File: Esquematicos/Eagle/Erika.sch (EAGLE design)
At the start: 12 parts

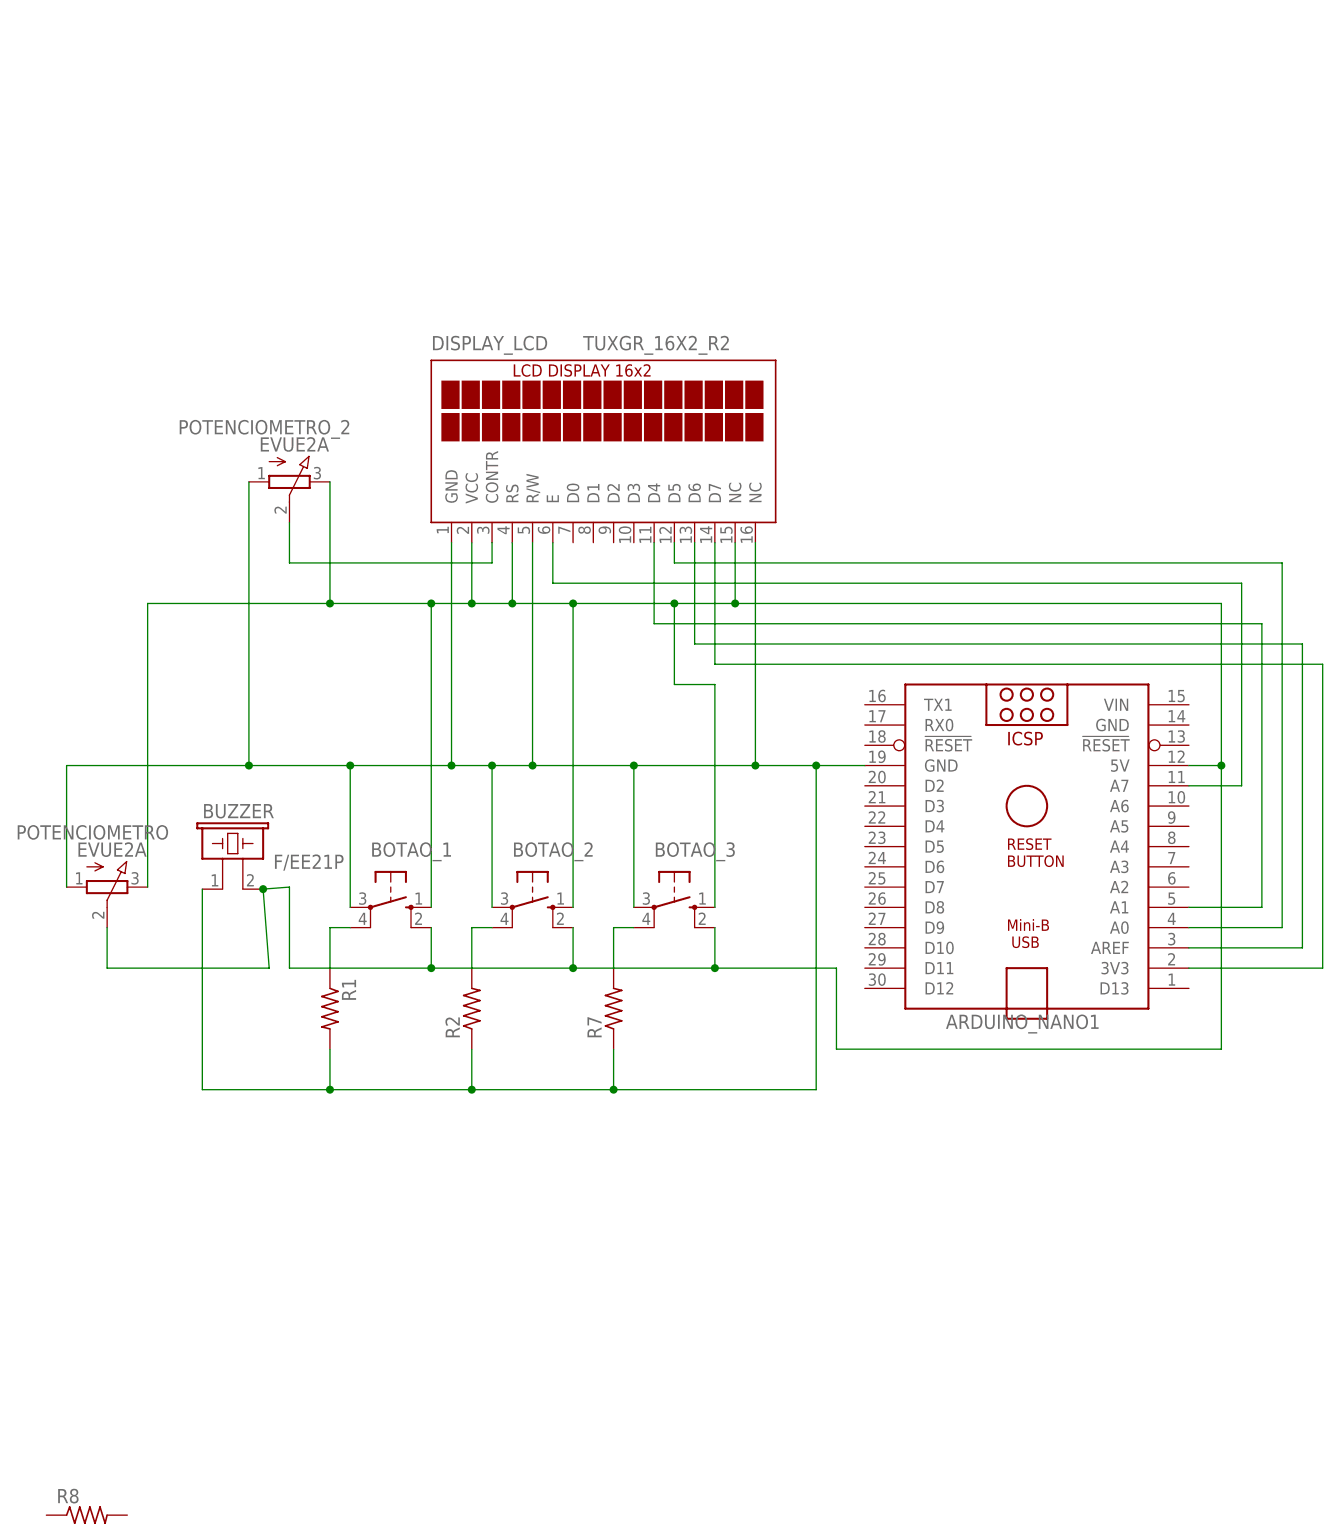
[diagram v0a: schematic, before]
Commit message: Correção do esquemático
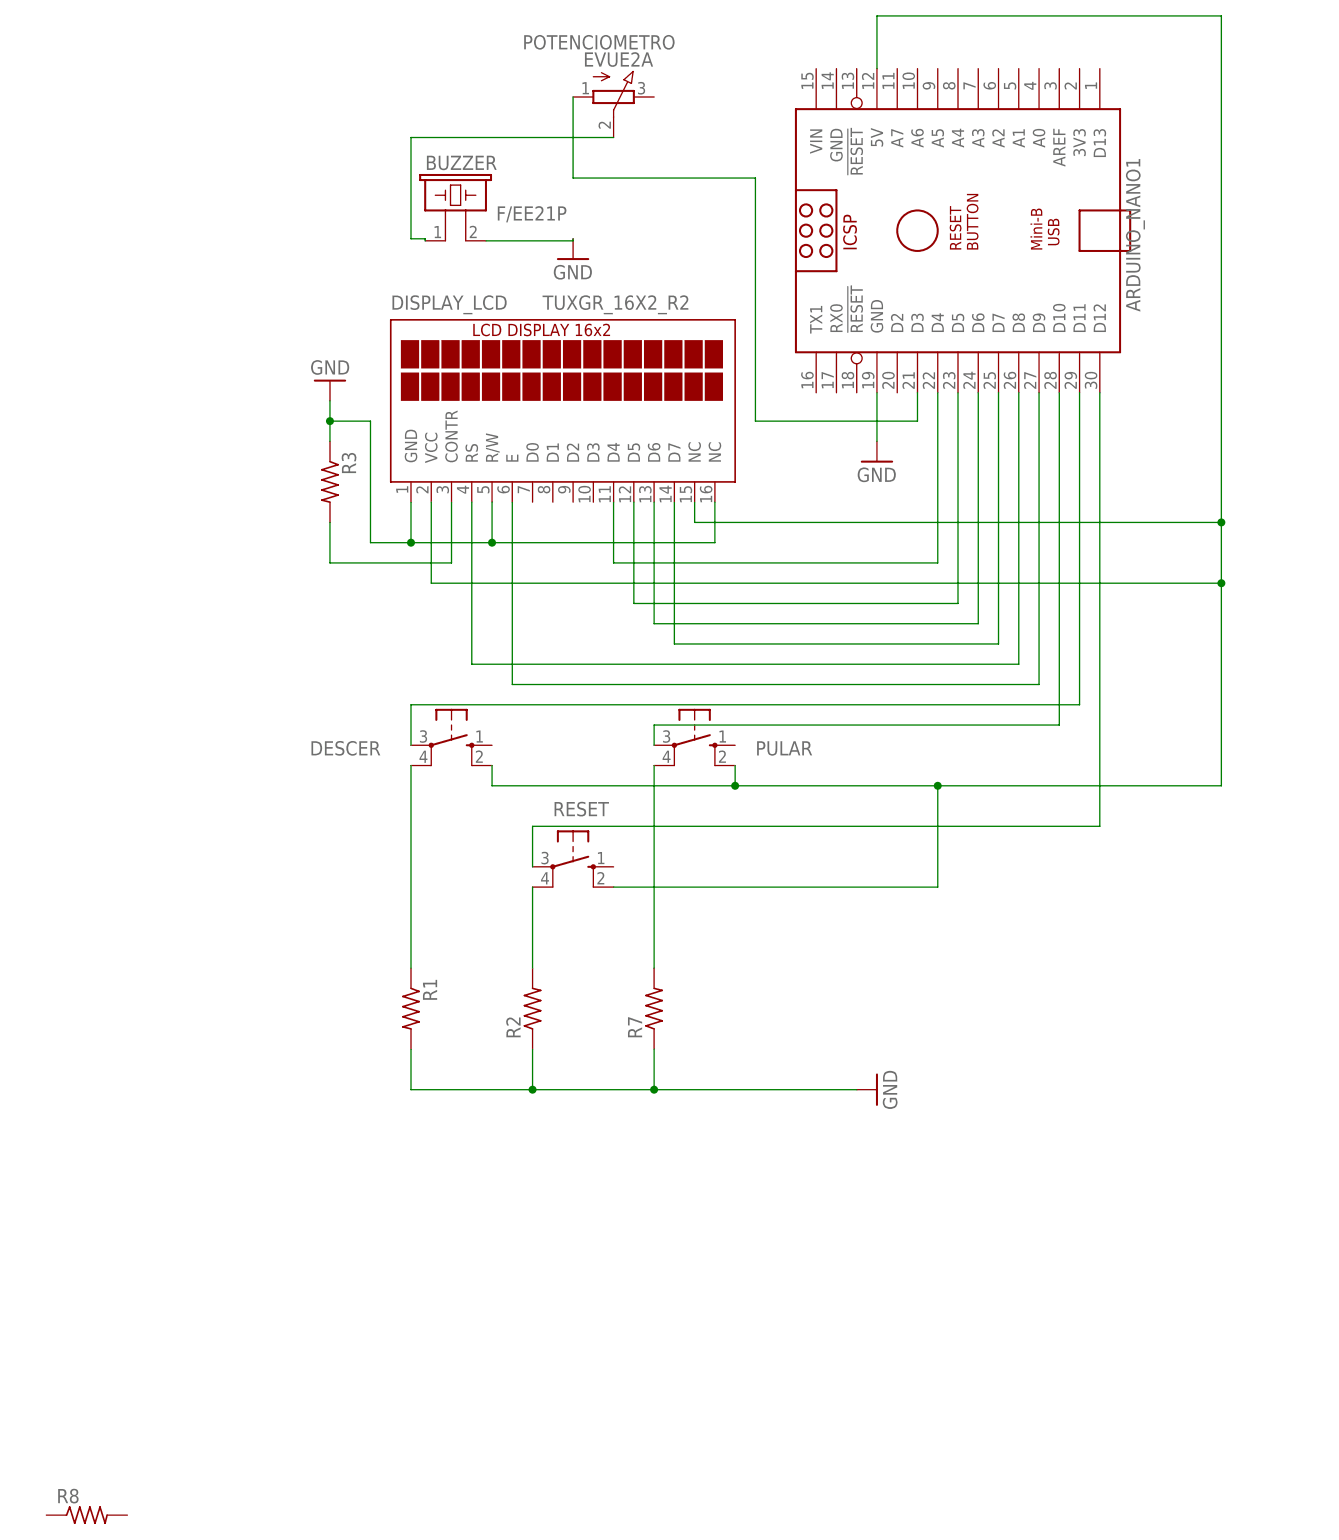
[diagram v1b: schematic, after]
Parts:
- removed BOTAO_1, BOTAO_2, BOTAO_3: (no value), switch-omron:10-XX
- removed POTENCIOMETRO_2: EVUE2A, pot:EVUE2A
- added DESCER, PULAR, RESET: (no value), switch-omron:10-XX
- added R3: (no value), rcl:R-US_0204/7
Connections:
- new net GND: ARDUINO_NANO1.GND@1, BUZZER.2, DISPLAY_LCD.GND, DISPLAY_LCD.NC@2, DISPLAY_LCD.R/W, R1.2, R2.1, R3.1, R7.1
- new net N$1: ARDUINO_NANO1.D4, DISPLAY_LCD.D4
- new net N$13: ARDUINO_NANO1.D7, DISPLAY_LCD.D7
- new net N$14: ARDUINO_NANO1.D8, DISPLAY_LCD.RS
- new net N$15: ARDUINO_NANO1.D9, DISPLAY_LCD.E
- new net N$16: ARDUINO_NANO1.D3, POTENCIOMETRO.A
- net N$10: now also PULAR.P1; no longer BOTAO_3.P1
- net N$11: now also R3.2; no longer POTENCIOMETRO_2.S
- net N$12: now also ARDUINO_NANO1.D6, DISPLAY_LCD.D6; no longer ARDUINO_NANO1.GND@1, BOTAO_1.P, BOTAO_2.P, BOTAO_3.P, BUZZER.1, DISPLAY_LCD.GND, DISPLAY_LCD.NC@2, DISPLAY_LCD.R/W, POTENCIOMETRO.A, POTENCIOMETRO_2.A, R1.2, R2.1, R7.1
- net N$2: now also DESCER.P1; no longer BOTAO_1.P1
- net N$3: now also ARDUINO_NANO1.D10, PULAR.P; no longer ARDUINO_NANO1.A7, DISPLAY_LCD.E
- net N$4: now also ARDUINO_NANO1.D11, DESCER.P; no longer ARDUINO_NANO1.A1, DISPLAY_LCD.D4
- net N$5: now also ARDUINO_NANO1.D12, RESET.P; no longer ARDUINO_NANO1.A0, DISPLAY_LCD.D5
- net N$6: now also BUZZER.1, POTENCIOMETRO.S; no longer ARDUINO_NANO1.AREF, DISPLAY_LCD.D6
- net N$7: now also ARDUINO_NANO1.D5, DISPLAY_LCD.D5; no longer ARDUINO_NANO1.3V3, DISPLAY_LCD.D7
- net N$8: now also RESET.P1; no longer BOTAO_2.P1
- net N$9: now also DESCER.S1, PULAR.S1, RESET.S1; no longer BOTAO_1.S, BOTAO_1.S1, BOTAO_2.S, BOTAO_2.S1, BOTAO_3.S, BOTAO_3.S1, BUZZER.2, DISPLAY_LCD.RS, POTENCIOMETRO.E, POTENCIOMETRO.S, POTENCIOMETRO_2.E
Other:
- moved on the sheet: ARDUINO_NANO1, BUZZER, DISPLAY_LCD, POTENCIOMETRO, R1, R2, R7
